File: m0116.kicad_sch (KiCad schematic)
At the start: 249 parts, among them J2 Conn_01x04_MountingPin, J3 Conn_01x04_MountingPin, Q1 Q_PMOS_GSD AO3401A, Q2 Q_NMOS_GSD 2N7002, Q3 Q_NMOS_GSD 2N7002, Q4 2N3904, SW1 SW_Push, U1 XC6206P332MR, U2 74AHCT1G125, U3 STM32F411RETx, U4 24LC64, U5 USBLC6-2SC6, Y1 8MHz

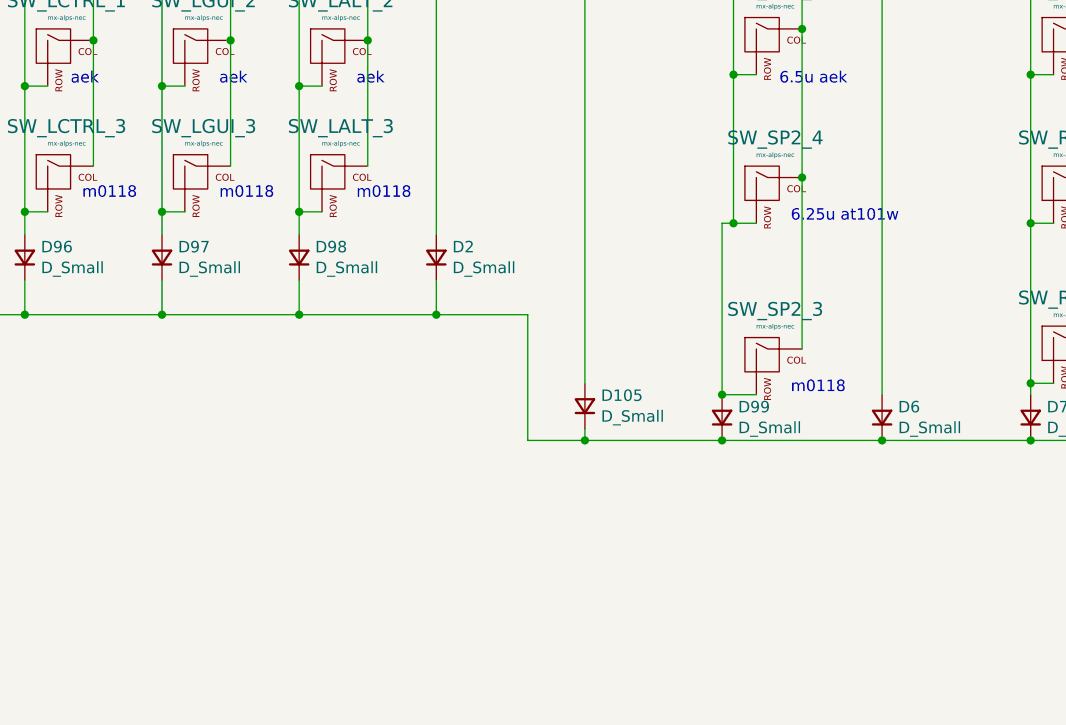
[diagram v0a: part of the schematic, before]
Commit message: update
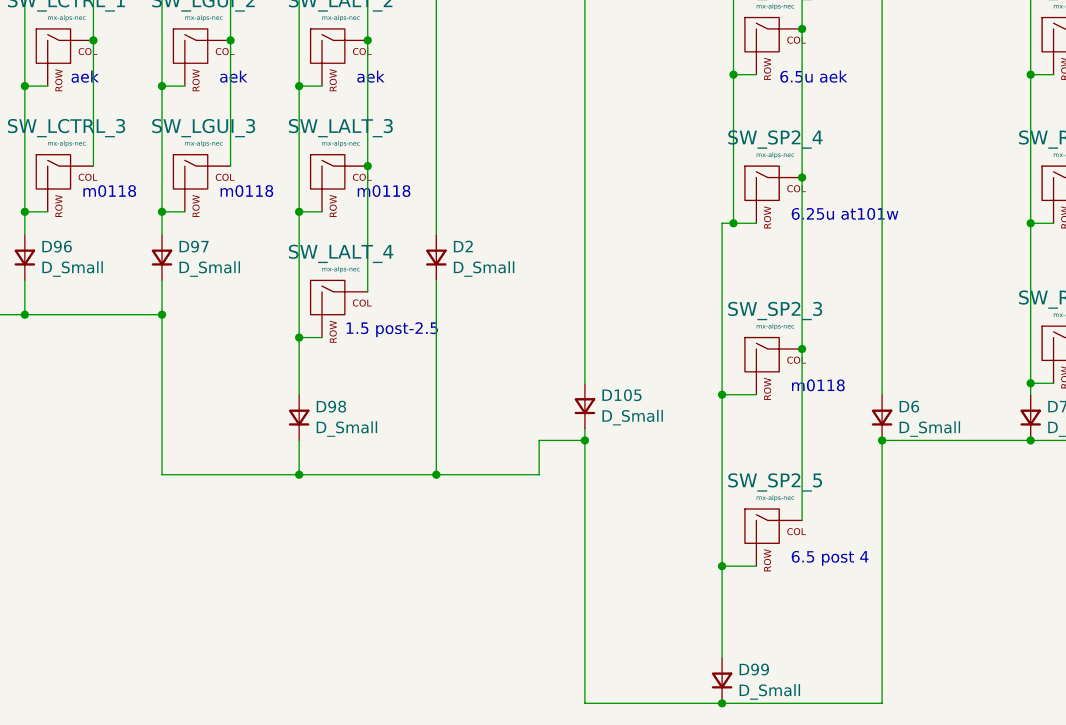
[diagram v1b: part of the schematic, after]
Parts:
- added SW_LALT_4, SW_SP2_5: mx-alps-nec, Alps_Only:ALPS-1U, symbol MX_Alps_Hybrid:mx-alps-nec
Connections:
- net COL3: now also SW_LALT_4.1 (COL)
- net COL6: now also SW_SP2_5.1 (COL)
- net at D99.2 (A), SW_SP2_1.2 (ROW), SW_SP2_2.2 (ROW)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: now also SW_SP2_5.2 (ROW)
- net at D98.2 (A), SW_LALT_1.2 (ROW), SW_LALT_2.2 (ROW)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: now also SW_LALT_4.2 (ROW)
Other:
- note added: "1.5 post-2.5"
- note added: "6.5 post 4"
- moved on the sheet: D98, D99

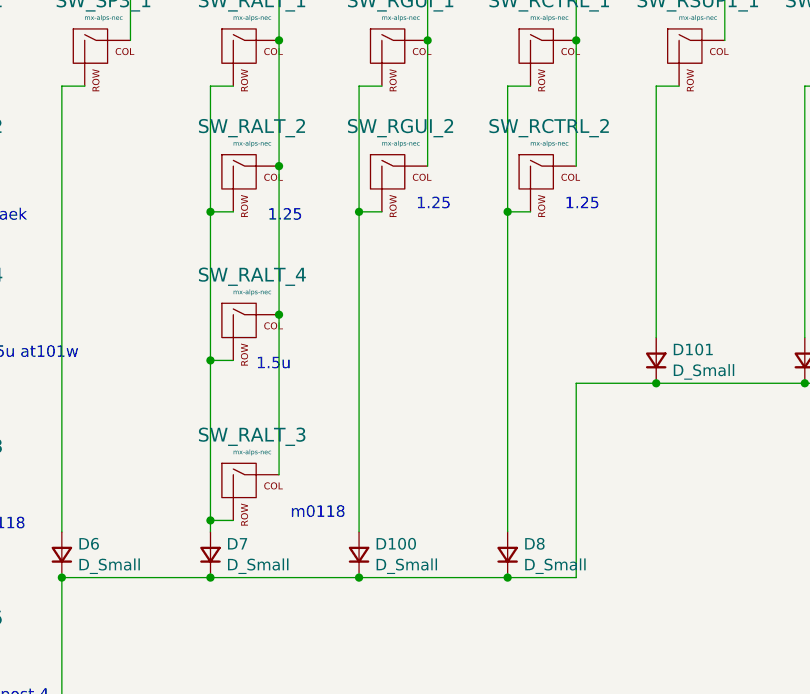
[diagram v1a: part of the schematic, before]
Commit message: update
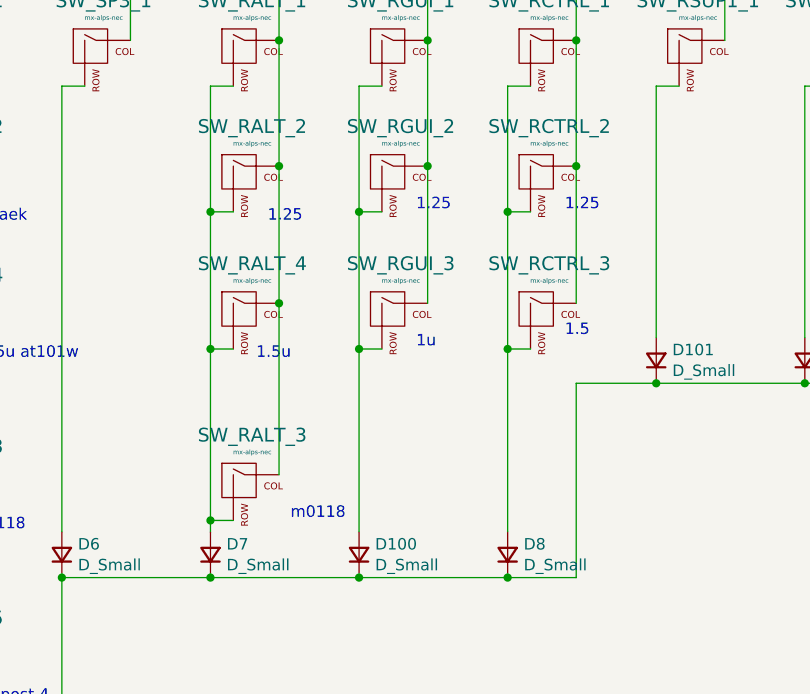
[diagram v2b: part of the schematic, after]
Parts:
- added SW_RCTRL_3, SW_RGUI_3: mx-alps-nec, Alps_Only:ALPS-1U, symbol MX_Alps_Hybrid:mx-alps-nec
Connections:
- net COL10: now also SW_RCTRL_3.1 (COL)
- net COL9: now also SW_RGUI_3.1 (COL)
- net at D100.2 (A), SW_RGUI_1.2 (ROW), SW_RGUI_2.2 (ROW): now also SW_RGUI_3.2 (ROW)
- net at D8.2 (A), SW_RCTRL_1.2 (ROW), SW_RCTRL_2.2 (ROW): now also SW_RCTRL_3.2 (ROW)
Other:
- note added: "1.5"
- note added: "1u"
- moved on the sheet: SW_RALT_4
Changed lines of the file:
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@@
   (junction (at 160.02 361.95) (diameter 0) (color 0 0 0 0)
   )
+  (junction (at 160.02 377.19) (diameter 0) (color 0 0 0 0)
+  )
   (junction (at 204.47 65.405) (diameter 0) (color 0 0 0 0)
   )
@@
   (junction (at 196.85 36.83) (diameter 0) (color 0 0 0 0)
   )
+  (junction (at 193.04 377.19) (diameter 0) (color 0 0 0 0)
+  )
   (junction (at 257.81 295.91) (diameter 0) (color 0 0 0 0)
   )
@@
   (junction (at 217.17 285.75) (diameter 1.016) (color 0 0 0 0)
   )
-  (junction (at 160.02 378.46) (diameter 0) (color 0 0 0 0)
-  )
   (junction (at 220.98 29.21) (diameter 0) (color 0 0 0 0)
   )
@@
   (junction (at 233.68 266.7) (diameter 1.016) (color 0 0 0 0)
   )
+  (junction (at 200.66 356.87) (diameter 0) (color 0 0 0 0)
+  )
   (junction (at 298.45 285.75) (diameter 1.016) (color 0 0 0 0)
   )
@@
   (junction (at 127 328.93) (diameter 0) (color 0 0 0 0)
   )
+  (junction (at 176.53 377.19) (diameter 0) (color 0 0 0 0)
+  )
   (junction (at 160.02 396.24) (diameter 0) (color 0 0 0 0)
   )
@@
   (junction (at 167.64 304.8) (diameter 0) (color 0 0 0 0)
   )
+  (junction (at 184.15 356.87) (diameter 0) (color 0 0 0 0)
+  )
   (junction (at 78.74 314.96) (diameter 0) (color 0 0 0 0)
   )
@@
   (junction (at 48.26 334.01) (diameter 0) (color 0 0 0 0)
   )
-  (junction (at 167.64 373.38) (diameter 0) (color 0 0 0 0)
-  )
   (junction (at 265.43 285.75) (diameter 1.016) (color 0 0 0 0)
   )
@@
   (junction (at 208.915 36.83) (diameter 0) (color 0 0 0 0)
   )
+  (junction (at 167.64 372.11) (diameter 0) (color 0 0 0 0)
+  )
   (junction (at 127 334.01) (diameter 1.016) (color 0 0 0 0)
   )
@@
     (stroke (width 0) (type default))
   )
+  (wire (pts (xy 176.53 377.19) (xy 179.07 377.19))
+    (stroke (width 0) (type default))
+  )
   (wire (pts (xy 77.47 118.11) (xy 88.9 118.11))
     (stroke (width 0) (type default))
@@
     (stroke (width 0) (type default))
   )
+  (wire (pts (xy 184.15 356.87) (xy 184.15 372.11))
+    (stroke (width 0) (type default))
+  )
   (wire (pts (xy 110.49 401.32) (xy 110.49 402.59))
     (stroke (width 0) (type default))
@@
     (stroke (width 0) (type default))
   )
-  (wire (pts (xy 160.02 378.46) (xy 160.02 396.24))
-    (stroke (width 0) (type default))
-  )
   (wire (pts (xy 210.82 160.02) (xy 210.82 156.21))
     (stroke (width 0) (type default))
@@
     (stroke (width 0) (type solid))
   )
-  (wire (pts (xy 160.02 378.46) (xy 162.56 378.46))
+  (wire (pts (xy 160.02 377.19) (xy 162.56 377.19))
     (stroke (width 0) (type default))
   )
@@
     (stroke (width 0) (type default))
   )
+  (wire (pts (xy 200.66 356.87) (xy 200.66 372.11))
+    (stroke (width 0) (type default))
+  )
   (wire (pts (xy 106.68 91.44) (xy 125.73 91.44))
     (stroke (width 0) (type default))
@@
     (stroke (width 0) (type default))
   )
+  (wire (pts (xy 193.04 361.95) (xy 193.04 377.19))
+    (stroke (width 0) (type default))
+  )
   (wire (pts (xy 236.22 307.34) (xy 236.22 306.07))
     (stroke (width 0) (type default))
@@
     (stroke (width 0) (type default))
   )
-  (wire (pts (xy 160.02 361.95) (xy 160.02 378.46))
+  (wire (pts (xy 160.02 361.95) (xy 160.02 377.19))
     (stroke (width 0) (type default))
   )
@@
     (stroke (width 0) (type default))
   )
-  (wire (pts (xy 167.64 373.38) (xy 167.64 391.16))
-    (stroke (width 0) (type default))
-  )
   (wire (pts (xy 33.02 347.98) (xy 35.56 347.98))
     (stroke (width 0) (type solid))
@@
     (stroke (width 0) (type default))
   )
-  (wire (pts (xy 167.64 356.87) (xy 167.64 373.38))
+  (wire (pts (xy 167.64 356.87) (xy 167.64 372.11))
     (stroke (width 0) (type default))
   )
@@
     (stroke (width 0) (type default))
   )
-  (wire (pts (xy 193.04 361.95) (xy 193.04 397.51))
-    (stroke (width 0) (type default))
-  )
   (wire (pts (xy 209.55 347.98) (xy 212.09 347.98))
     (stroke (width 0) (type solid))
@@
     (stroke (width 0) (type solid))
   )
+  (wire (pts (xy 160.02 377.19) (xy 160.02 396.24))
+    (stroke (width 0) (type default))
+  )
   (wire (pts (xy 143.51 168.91) (xy 143.51 167.64))
     (stroke (width 0) (type default))
@@
     (stroke (width 0) (type solid))
   )
+  (wire (pts (xy 167.64 372.11) (xy 167.64 391.16))
+    (stroke (width 0) (type default))
+  )
   (wire (pts (xy 143.51 347.98) (xy 143.51 397.51))
     (stroke (width 0) (type default))
@@
     (stroke (width 0) (type default))
   )
-  (wire (pts (xy 176.53 361.95) (xy 176.53 397.51))
+  (wire (pts (xy 176.53 361.95) (xy 176.53 377.19))
     (stroke (width 0) (type default))
   )
@@
     (stroke (width 0) (type solid))
   )
+  (wire (pts (xy 176.53 377.19) (xy 176.53 397.51))
+    (stroke (width 0) (type default))
+  )
   (wire (pts (xy 125.73 378.46) (xy 125.73 397.51))
     (stroke (width 0) (type default))
@@
     (stroke (width 0) (type solid))
   )
+  (wire (pts (xy 193.04 377.19) (xy 195.58 377.19))
+    (stroke (width 0) (type default))
+  )
   (wire (pts (xy 186.69 194.31) (xy 194.31 194.31))
     (stroke (width 0) (type solid))
@@
     (stroke (width 0) (type solid))
   )
+  (wire (pts (xy 193.04 377.19) (xy 193.04 397.51))
+    (stroke (width 0) (type default))
+  )
   (wire (pts (xy 176.53 314.96) (xy 193.04 314.96))
     (stroke (width 0) (type solid))
@@
     (effects (font (size 1.27 1.27)) (justify left bottom))
   )
+  (text "1.5" (at 199.39 375.92 0)
+    (effects (font (size 1.27 1.27)) (justify left bottom))
+  )
   (text "m0118" (at 54.61 375.92 0)
     (effects (font (size 1.27 1.27)) (justify left bottom))
@@
     (effects (font (size 1.27 1.27)) (justify left bottom))
   )
-  (text "1.5u\n" (at 165.1 379.73 0)
+  (text "1u" (at 182.88 377.19 0)
+    (effects (font (size 1.27 1.27)) (justify left bottom))
+  )
+  (text "1.5u\n" (at 165.1 378.46 0)
     (effects (font (size 1.27 1.27)) (justify left bottom))
   )
@@
     )
   )
+  (symbol (lib_id "MX_Alps_Hybrid:mx-alps-nec") (at 196.85 373.38 0) (unit 1)
+    (in_bom yes) (on_board yes) (dnp no)
+    (property "Reference" "SW_RCTRL_3" (at 197.6882 367.7158 0)
+      (effects (font (size 1.524 1.524)))
+    )
+    (property "Value" "mx-alps-nec" (at 197.6882 369.5954 0)
+      (effects (font (size 0.508 0.508)))
+    )
+    (property "Footprint" "Alps_Only:ALPS-1U" (at 180.975 374.015 0)
+      (effects (font (size 1.524 1.524)) hide)
+    )
+    (property "Datasheet" "" (at 180.975 374.015 0)
+      (effects (font (size 1.524 1.524)) hide)
+    )
+    (pin "1")
+    (pin "2")
+    (instances
+      (project "m0116"
+        (path "/151da08b-0979-4785-a9bf-6fa9b165d629"
+          (reference "SW_RCTRL_3") (unit 1)
+        )
+      )
+    )
+  )
   (symbol (lib_id "MX_Alps_Hybrid:mx-alps-nec") (at 294.64 306.07 0) (unit 1)
     (in_bom yes) (on_board yes) (dnp no)
@@
     )
   )
-  (symbol (lib_id "MX_Alps_Hybrid:mx-alps-nec") (at 163.83 374.65 0) (unit 1)
+  (symbol (lib_id "MX_Alps_Hybrid:mx-alps-nec") (at 163.83 373.38 0) (unit 1)
     (in_bom yes) (on_board yes) (dnp no)
-    (property "Reference" "SW_RALT_4" (at 164.6682 368.9858 0)
+    (property "Reference" "SW_RALT_4" (at 164.6682 367.7158 0)
       (effects (font (size 1.524 1.524)))
     )
-    (property "Value" "mx-alps-nec" (at 164.6682 370.8654 0)
+    (property "Value" "mx-alps-nec" (at 164.6682 369.5954 0)
       (effects (font (size 0.508 0.508)))
     )
-    (property "Footprint" "Alps_Only:ALPS-1U" (at 147.955 375.285 0)
+    (property "Footprint" "Alps_Only:ALPS-1U" (at 147.955 374.015 0)
       (effects (font (size 1.524 1.524)) hide)
     )
-    (property "Datasheet" "" (at 147.955 375.285 0)
+    (property "Datasheet" "" (at 147.955 374.015 0)
       (effects (font (size 1.524 1.524)) hide)
     )
@@
         )
       )
+    )
+  )
+  (symbol (lib_id "MX_Alps_Hybrid:mx-alps-nec") (at 180.34 373.38 0) (unit 1)
+    (in_bom yes) (on_board yes) (dnp no)
+    (property "Reference" "SW_RGUI_3" (at 181.1782 367.7158 0)
+      (effects (font (size 1.524 1.524)))
+    )
+    (property "Value" "mx-alps-nec" (at 181.1782 369.5954 0)
+      (effects (font (size 0.508 0.508)))
+    )
+    (property "Footprint" "Alps_Only:ALPS-1U" (at 164.465 374.015 0)
+      (effects (font (size 1.524 1.524)) hide)
+    )
+    (property "Datasheet" "" (at 164.465 374.015 0)
+      (effects (font (size 1.524 1.524)) hide)
+    )
+    (pin "1")
+    (pin "2")
+    (instances
+      (project "m0116"
+        (path "/151da08b-0979-4785-a9bf-6fa9b165d629"
+          (reference "SW_RGUI_3") (unit 1)
+        )
+      )
